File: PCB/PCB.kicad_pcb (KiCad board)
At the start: 2 copper layers, 30.5 x 25.5 mm, 23 parts, among them U1 STM32G031F6P6, U2 A7106, U3 HT7333-3.3V, Y1 16MHz

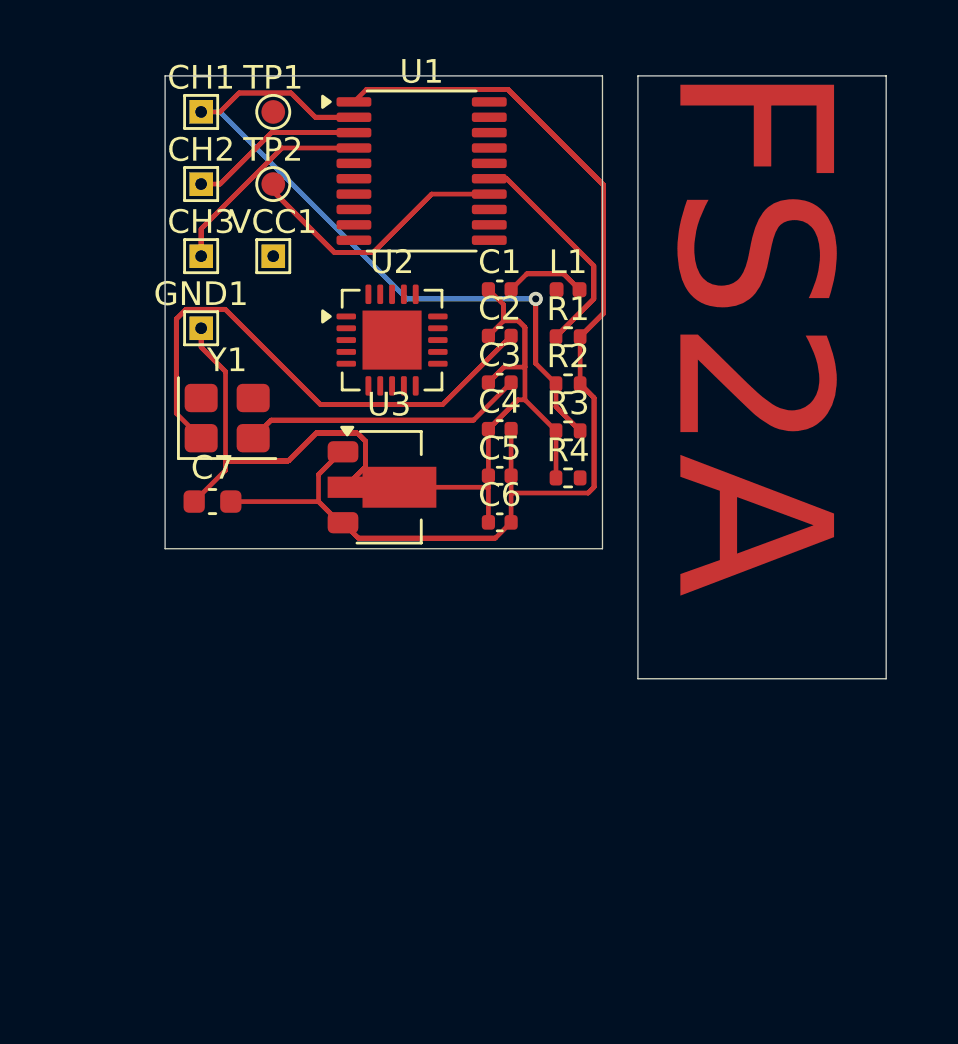
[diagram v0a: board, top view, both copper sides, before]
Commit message: fix: Migrate symbol
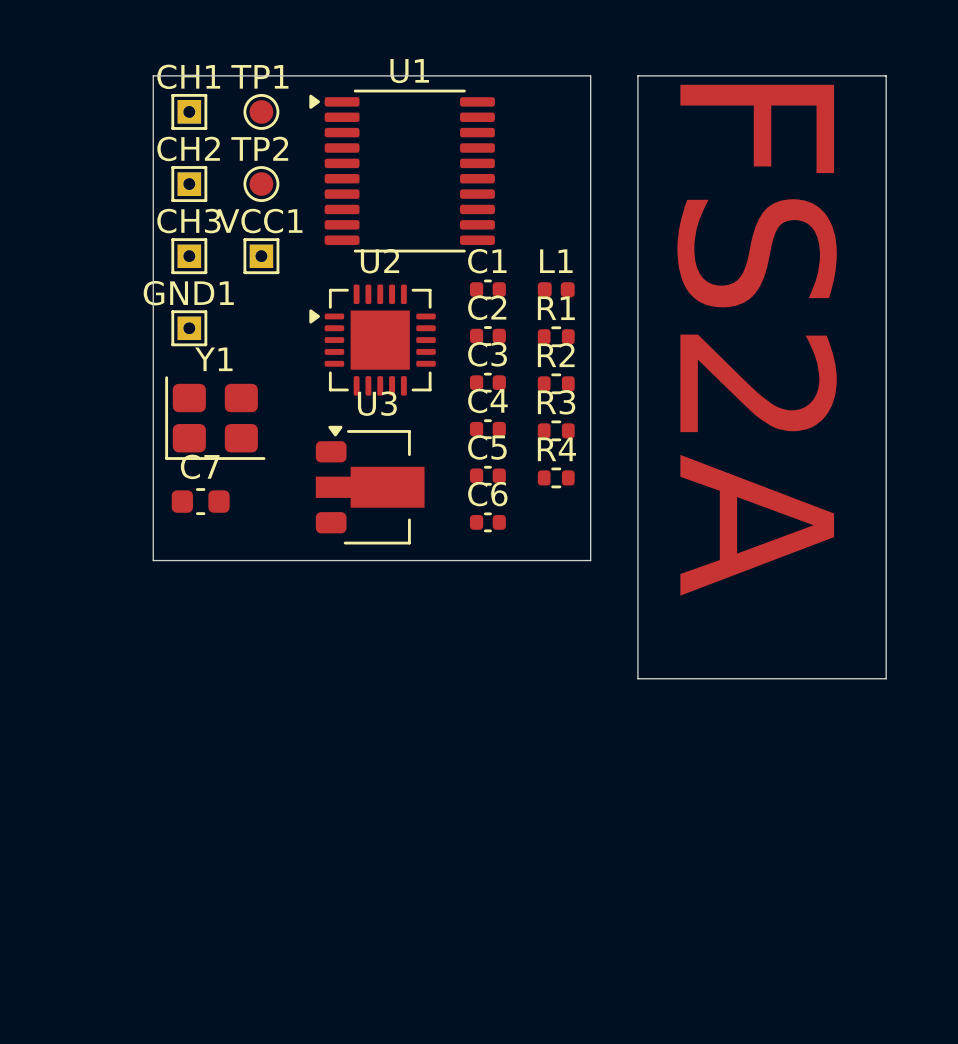
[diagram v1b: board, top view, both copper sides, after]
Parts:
- moved C1 0.50 mm to (165.7, 68.0)
- moved C2 0.50 mm to (165.7, 70.0)
- moved C3 0.50 mm to (165.7, 72.0)
- moved C4 0.50 mm to (165.7, 73.9)
- moved C5 0.50 mm to (165.7, 75.9)
- moved C6 0.50 mm to (165.7, 77.9)
- moved C7 0.50 mm to (153.5, 77.0)
- moved CH1 0.50 mm to (153.0, 60.5)
- moved CH2 0.50 mm to (153.0, 63.6)
- moved CH3 0.50 mm to (153.0, 66.6)
- moved GND1 0.50 mm to (153.0, 69.7)
- moved L1 0.50 mm to (168.5, 68.0)
- moved R1 0.50 mm to (168.5, 70.0)
- moved R2 0.50 mm to (168.5, 72.0)
- moved R3 0.50 mm to (168.5, 74.0)
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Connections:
- C7 pad 2: /+3.3V -> /VCC1
- CH1 pad 1: /ADC -> /CH1
- GND1 pad 1: /GND -> Net-(U3-GND)
- R2 pad 2: /+3.3V -> /VCC1
- U1 pad 1: /+3.3V -> Net-(U1-VDD)
- U1 pad 14: /SWCLK -> unconnected-(U1-PA14-Pad14)
- U1 pad 15: /NRST -> unconnected-(U1-NRST-Pad15)
- U1 pad 16: /CSN -> unconnected-(U1-PB0-Pad16)
- U1 pad 2: /ADC -> unconnected-(U1-PA0-Pad2)
- U1 pad 3: /CH2 -> unconnected-(U1-PA1-Pad3)
- U1 pad 4: /CH3 -> unconnected-(U1-PA2-Pad4)
- U1 pad 5: /CE -> unconnected-(U1-PA3-Pad5)
- U1 pad 6: /IRQ -> unconnected-(U1-PA4-Pad6)
- U1 pad 7: /SCK -> unconnected-(U1-PA5-Pad7)
- U1 pad 8: /MISO -> unconnected-(U1-PA6-Pad8)
- U1 pad 9: /MOSI -> unconnected-(U1-PA7-Pad9)
- U3 pad 1: /+3.3V -> Net-(U3-VIN)
- U3 pad 2: /GND -> Net-(U3-GND)
- U3 pad 3: /+3.3V -> Net-(U1-VDD)
- VCC1 pad 1: unconnected-(VCC1-Pad1) -> Net-(U3-VIN)
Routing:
- net /+3.3V: track 102.5 -> 0.00 mm
- net /GND: track 85.7 -> 0.00 mm
- net /ADC: track 58.2 -> 0.00 mm, vias 1 -> 0
- net /XC1: track 43.9 -> 0.00 mm
- net /SWCLK: track 30.5 -> 0.00 mm
- net /NRST: track 24.4 -> 0.00 mm
- net /XC2: track 21.5 -> 0.00 mm
- net /CH3: track 16.2 -> 0.00 mm
- net /CH2: track 13.9 -> 0.00 mm
- net /ANT: track 5.96 -> 0.00 mm
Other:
- board size 30.5 x 25.5 mm -> 31 x 25.5 mm

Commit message: feat: Update PCB
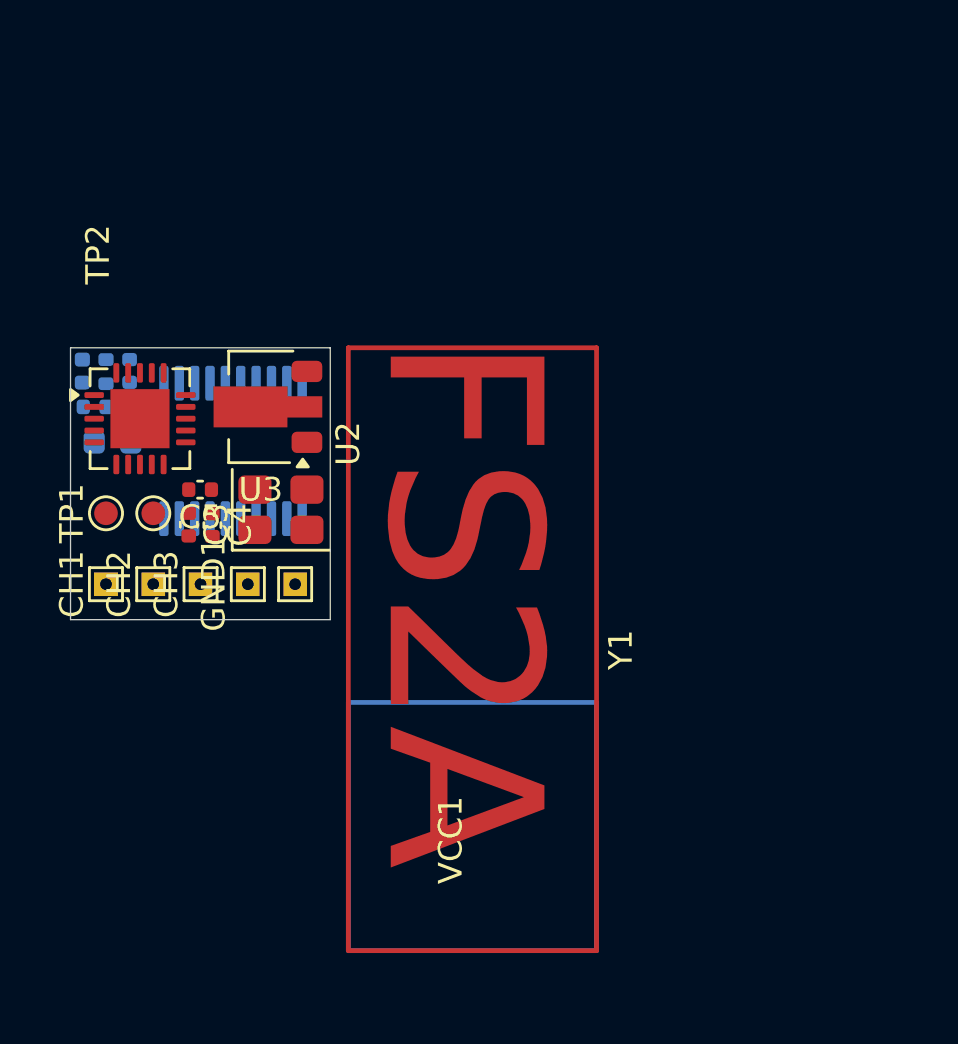
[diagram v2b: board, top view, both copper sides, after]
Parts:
- removed C1: 2.7pF, Capacitor_SMD:C_0402_1005Metric
- removed R2: 10k, Resistor_SMD:R_0402_1005Metric
- removed R3: 1.8k, Resistor_SMD:R_0402_1005Metric
- removed R4: 22k, Resistor_SMD:R_0402_1005Metric
- C2, C6, C7, L1, R1, U1: moved to B.Cu
- moved L1 20.3 mm to (148.5, 71.5), turned to -90 degrees
- moved CH1 20.3 mm to (149.5, 80.5), turned to 90 degrees
- moved R1 19.1 mm to (149.5, 71.5), turned to -90 degrees
- moved TP1 18.2 mm to (149.5, 77.5), turned to 90 degrees
- moved CH2 17.0 mm to (151.5, 80.5), turned to 90 degrees
- moved C2 16.9 mm to (149.0, 73.0)
- moved C6 16.5 mm to (150.5, 71.5), turned to 90 degrees
- moved TP2 14.7 mm to (151.5, 77.5), turned to 90 degrees
- moved C3 14.0 mm to (153.0, 78.0), turned to -90 degrees
- moved U1 14.0 mm to (154.9, 74.9), turned to -90 degrees
- moved VCC1 13.9 mm to (157.5, 80.5)
- moved CH3 13.9 mm to (153.5, 80.5), turned to 90 degrees
- moved C4 12.3 mm to (154.0, 78.0), turned to -90 degrees
- moved C5 12.2 mm to (153.5, 76.5), turned to 180 degrees
- moved GND1 11.1 mm to (155.5, 80.5), turned to 90 degrees
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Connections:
- net /XC1 renamed Net-(C2-Pad2)
- C2 pad 1: /GND -> Net-(U2-XI)
- C3 pad 1: /GND -> Net-(C3-Pad1)
- C3 pad 2: /XC2 -> Net-(U2-XO)
- C4 pad 1: /GND -> Net-(U2-DVDD)
- C4 pad 2: /+3.3V -> Net-(U1-VDD)
- C5 pad 1: /GND -> Net-(U1-VSS)
- C5 pad 2: /+3.3V -> Net-(U2-REGI)
- C6 pad 1: /GND -> Net-(U1-VSS)
- C6 pad 2: /+3.3V -> Net-(U2-BPBG)
- C7 pad 1: /GND -> Net-(C7-Pad1)
- C7 pad 2: /VCC1 -> Net-(U3-VIN)
- CH1 pad 1: /CH1 -> Net-(U1-PA0)
- CH2 pad 1: /CH2 -> Net-(U1-PA1)
- CH3 pad 1: /CH3 -> Net-(U1-PA2)
- GND1 pad 1: Net-(U3-GND) -> Net-(U1-VSS)
- L1 pad 1: unconnected-(L1-Pad1) -> Net-(U2-RFO)
- L1 pad 2: /ANT -> unconnected-(L1-Pad2)
- R1 pad 1: /NRST -> Net-(U1-NRST)
- R1 pad 2: /+3.3V -> Net-(U2-DVDD)
- TP1 pad 1: /SWDIO -> Net-(U1-PA13)
- TP2 pad 1: /SWCLK -> Net-(U1-PA14)
- U1 pad 13: unconnected-(U1-PA13-Pad13) -> Net-(U1-PA13)
- U1 pad 14: unconnected-(U1-PA14-Pad14) -> Net-(U1-PA14)
- U1 pad 15: unconnected-(U1-NRST-Pad15) -> Net-(U1-NRST)
- U1 pad 16: unconnected-(U1-PB0-Pad16) -> Net-(U1-PB0)
- U1 pad 2: unconnected-(U1-PA0-Pad2) -> Net-(U1-PA0)
- U1 pad 20: unconnected-(U1-VSS-Pad20) -> Net-(U1-VSS)
- U1 pad 3: unconnected-(U1-PA1-Pad3) -> Net-(U1-PA1)
- U1 pad 4: unconnected-(U1-PA2-Pad4) -> Net-(U1-PA2)
- U1 pad 5: unconnected-(U1-PA3-Pad5) -> Net-(U1-PA3)
- U1 pad 7: unconnected-(U1-PA5-Pad7) -> Net-(U1-PA5)
- U1 pad 8: unconnected-(U1-PA6-Pad8) -> Net-(U1-PA6)
- U1 pad 9: unconnected-(U1-PA7-Pad9) -> Net-(U1-PA7)
- U2 pad 10: unconnected-(U2-VDA3-Pad10) -> Net-(U2-DVDD)
- U2 pad 11: unconnected-(U2-SCS-Pad11) -> Net-(U1-PA3)
- U2 pad 12: unconnected-(U2-SCK-Pad12) -> Net-(U1-PA5)
- U2 pad 13: unconnected-(U2-DVDD-Pad13) -> Net-(U2-DVDD)
- U2 pad 14: unconnected-(U2-SDIO-Pad14) -> Net-(U1-PA6)
- U2 pad 15: unconnected-(U2-GND-Pad15) -> Net-(U1-VSS)
- U2 pad 16: unconnected-(U2-GIO1-Pad16) -> Net-(U1-PA7)
- U2 pad 17: unconnected-(U2-GIO2-Pad17) -> Net-(U1-PB0)
- U2 pad 19: unconnected-(U2-REGI-Pad19) -> Net-(U2-REGI)
- U2 pad 2: unconnected-(U2-BPBG-Pad2) -> Net-(U2-BPBG)
- U2 pad 20: unconnected-(U2-VDA1-Pad20) -> Net-(U2-DVDD)
- U2 pad 4: unconnected-(U2-RFO-Pad4) -> Net-(U2-RFO)
- U2 pad 5: unconnected-(U2-VDA2-Pad5) -> Net-(U2-DVDD)
- U2 pad 7: unconnected-(U2-GND-Pad7) -> Net-(U1-VSS)
- U2 pad 8: unconnected-(U2-XI-Pad8) -> Net-(U2-XI)
- U2 pad 9: unconnected-(U2-XO-Pad9) -> Net-(U2-XO)
- U3 pad 2: Net-(U3-GND) -> Net-(U1-VSS)
- U3 pad 3: Net-(U1-VDD) -> Net-(U2-DVDD)
- VCC1 pad 1: Net-(U3-VIN) -> Net-(C7-Pad1)
- Y1 pad 2: /XC2 -> Net-(C3-Pad1)
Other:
- board size 31 x 25.5 mm -> 11 x 11.5 mm
